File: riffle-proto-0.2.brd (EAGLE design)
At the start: 62.2 x 18 mm, 15 parts

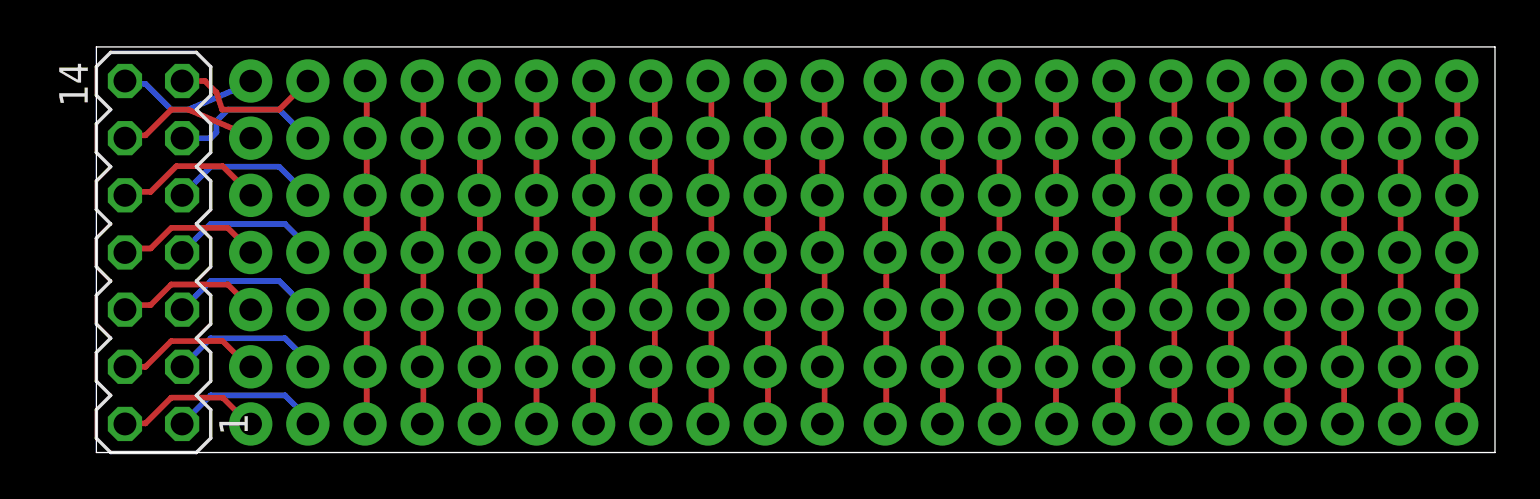
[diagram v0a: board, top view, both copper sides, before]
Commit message: update
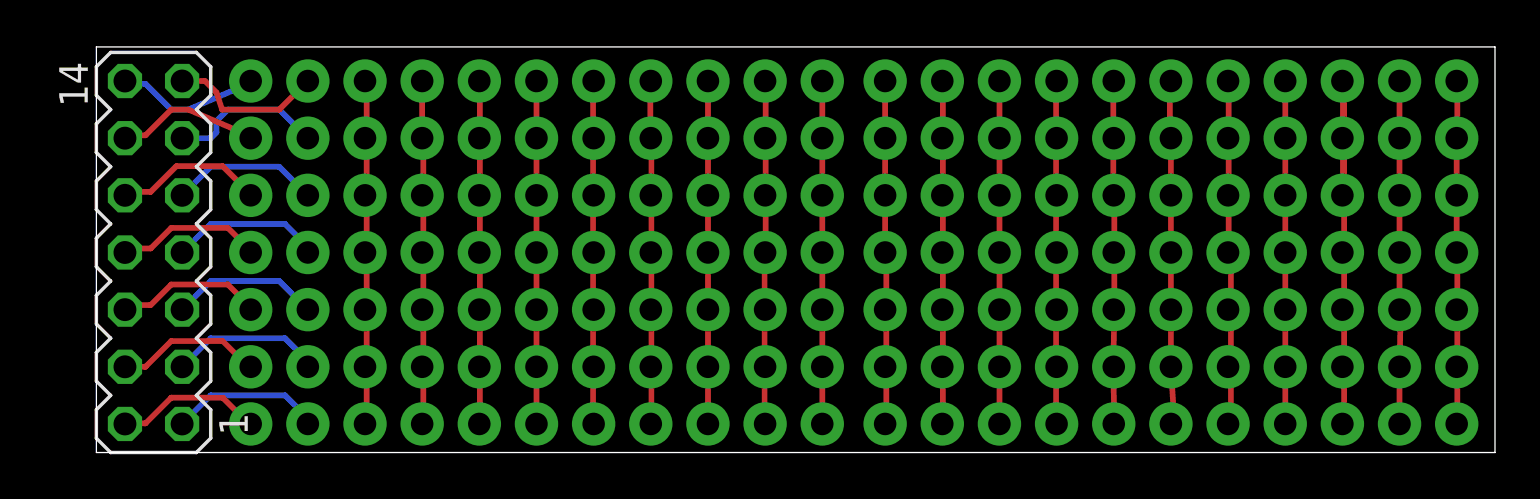
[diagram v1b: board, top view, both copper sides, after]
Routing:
- net N$44: track 15.6 -> 20.2 mm
- net N$20: track 16.5 -> 15.3 mm
- net N$40: track 16.5 -> 15.4 mm
- net N$21: track 16.2 -> 15.2 mm
- net N$41: track 16.2 -> 15.4 mm
- net N$22: track 16.0 -> 15.4 mm
- net N$43: track 15.8 -> 15.3 mm
